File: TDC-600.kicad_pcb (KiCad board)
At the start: 2 copper layers, 99.9 x 64 mm, 32 parts, among them J1 MSXCART1, J2 Conn_01x03_Male, J3 Conn_01x03_Male, J4 Conn_01x03_Male, J5 Conn_01x03_Male, J6 FDD Connector, J7 ROM_SWITCH, SW1 SW_Push, U1 AT28C256, U2 74LS04, U3 74LS138, U4 WDC37C65, Y1 16Mhz

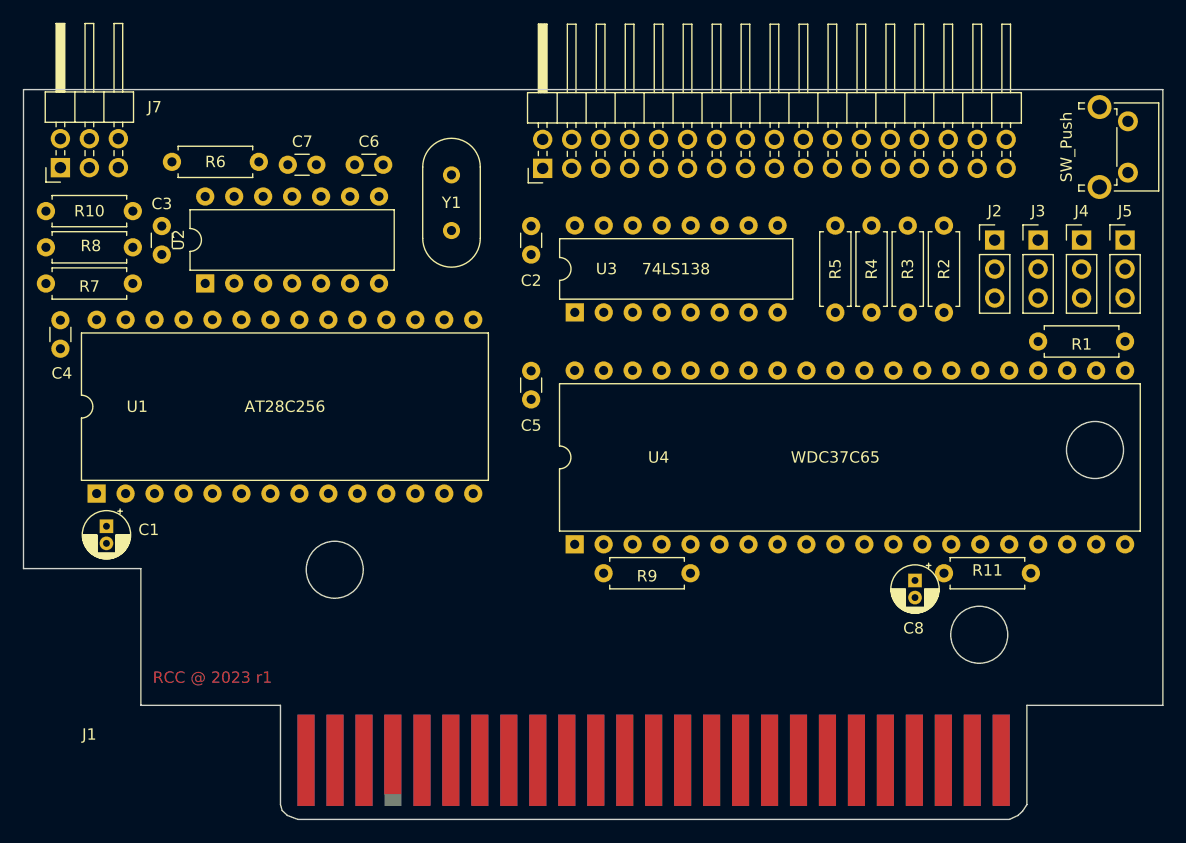
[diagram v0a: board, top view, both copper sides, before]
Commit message: Routing Release 1.0
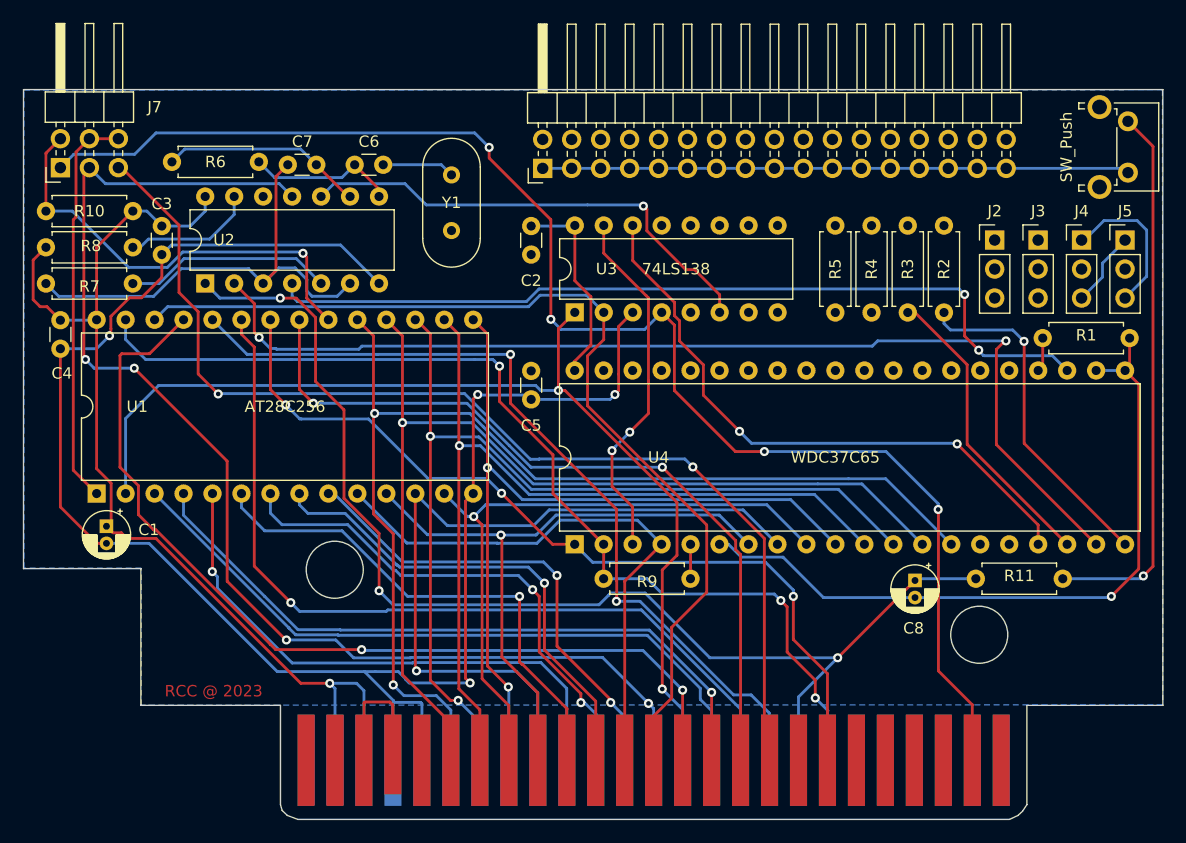
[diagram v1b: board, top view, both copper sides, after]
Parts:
- J1: footprint Roni Footprints:MSX_CART_SW_Official_3Holes -> Roni_Footprints:MSX_CART_SW_Official
- moved R1 8.03 mm to (128.5, 48.5), turned to 180 degrees
- moved R11 2.84 mm to (122.7, 69.6)
- moved R9 0.48 mm to (82.4, 69.6)
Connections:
- J1 pad 41: Net-(J1-Pad41) -> GNDREF
- J1 pad 43: Net-(J1-Pad41) -> GNDREF
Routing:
- net GNDREF: track 0.00 -> 268.6 mm, vias 0 -> 5
- net +5V: track 0.00 -> 138.2 mm, vias 0 -> 1
- net /SLTSL: track 0.00 -> 125.7 mm, vias 0 -> 4
- net A14: track 0.00 -> 109.1 mm, vias 0 -> 4
- net /RESET: track 0.00 -> 106.1 mm, vias 0 -> 3
- net D7: track 0.00 -> 99.0 mm, vias 0 -> 2
- net A15: track 0.00 -> 96.6 mm, vias 0 -> 2
- net WDRST: track 0.00 -> 93.7 mm, vias 0 -> 2
- net A12: track 0.00 -> 92.0 mm, vias 0 -> 2
- net D6: track 0.00 -> 91.0 mm, vias 0 -> 1
- net /WR: track 0.00 -> 89.5 mm, vias 0 -> 3
- net A13: track 0.00 -> 87.0 mm
- net D5: track 0.00 -> 86.0 mm, vias 0 -> 2
- net A8: track 0.00 -> 81.8 mm, vias 0 -> 2
- net D4: track 0.00 -> 79.6 mm, vias 0 -> 1
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- added copper zone on B.Cu, net GNDREF
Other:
- outline, holes or cut-outs redrawn
